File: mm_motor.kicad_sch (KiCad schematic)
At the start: 1 part, among them M1 N20_encoder

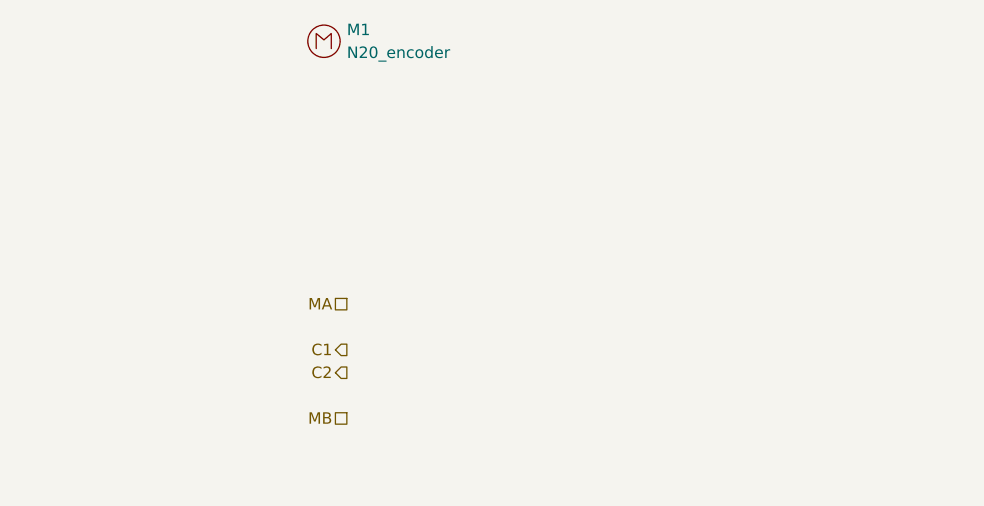
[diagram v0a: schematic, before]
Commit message: TP3
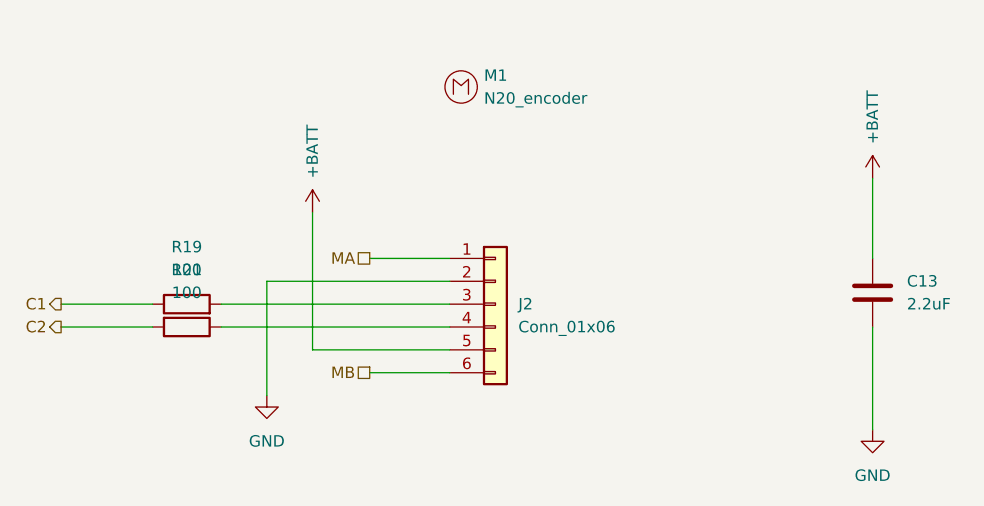
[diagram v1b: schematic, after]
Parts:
- added C13: 2.2uF, Capacitor_SMD:C_0603_1608Metric, symbol Device:C
- added J2: Conn_01x06, Connector_PinHeader_2.54mm:PinHeader_1x06_P2.54mm_Vertical, symbol Connector_Generic:Conn_01x06
- added R19, R21: 100, Resistor_SMD:R_0603_1608Metric, symbol Device:R
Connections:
- net C1: now also R19.1
- net C2: now also R21.2
- net MA: now also J2.1 (Pin_1)
- net MB: now also J2.6 (Pin_6)
- new net: J2.4 (Pin_4), R21.1
- new net: J2.3 (Pin_3), R19.2
- new net +BATT: C13.1, J2.5 (Pin_5)
- new net GND: C13.2, J2.2 (Pin_2)
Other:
- moved on the sheet: M1

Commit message: save
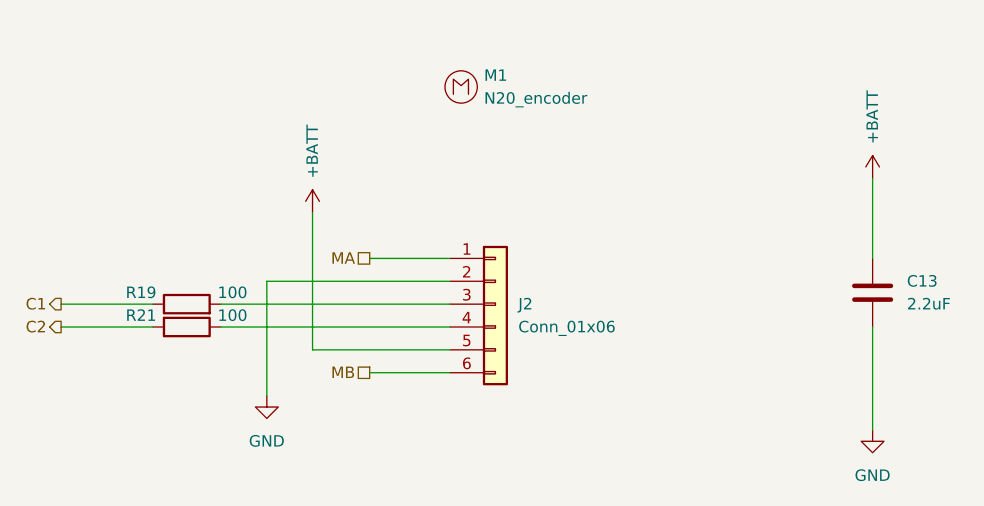
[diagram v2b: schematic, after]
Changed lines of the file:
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@@
   )
   (symbol (lib_id "Device:R") (at 100.33 88.9 270) (unit 1)
-    (in_bom yes) (on_board yes) (dnp no) (fields_autoplaced)
-    (property "Reference" "R21" (at 100.33 82.55 90)
-      (effects (font (size 1.27 1.27)))
-    )
-    (property "Value" "100" (at 100.33 85.09 90)
+    (in_bom yes) (on_board yes) (dnp no)
+    (property "Reference" "R21" (at 95.25 87.63 90)
+      (effects (font (size 1.27 1.27)))
+    )
+    (property "Value" "100" (at 105.41 87.63 90)
       (effects (font (size 1.27 1.27)))
     )
@@
         )
         (path "/d8fa4cba-2469-4231-847f-065b6b829f44/3975acd0-18ad-47bc-9ce1-d8c4d864aafe"
-          (reference "R15") (unit 1)
+          (reference "R22") (unit 1)
         )
       )
@@
         )
         (path "/d8fa4cba-2469-4231-847f-065b6b829f44/3975acd0-18ad-47bc-9ce1-d8c4d864aafe"
-          (reference "C12") (unit 1)
+          (reference "C14") (unit 1)
         )
       )
@@
   )
   (symbol (lib_id "Device:R") (at 100.33 86.36 90) (unit 1)
-    (in_bom yes) (on_board yes) (dnp no) (fields_autoplaced)
-    (property "Reference" "R19" (at 100.33 80.01 90)
-      (effects (font (size 1.27 1.27)))
-    )
-    (property "Value" "100" (at 100.33 82.55 90)
+    (in_bom yes) (on_board yes) (dnp no)
+    (property "Reference" "R19" (at 95.25 85.09 90)
+      (effects (font (size 1.27 1.27)))
+    )
+    (property "Value" "100" (at 105.41 85.09 90)
       (effects (font (size 1.27 1.27)))
     )
@@
         )
         (path "/d8fa4cba-2469-4231-847f-065b6b829f44/3975acd0-18ad-47bc-9ce1-d8c4d864aafe"
-          (reference "R14") (unit 1)
-        )
-      )
+          (reference "R20") (unit 1)
+        )
+      )
